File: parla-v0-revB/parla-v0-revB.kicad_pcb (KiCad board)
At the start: 2 copper layers, 80 x 80 mm, 25 parts, among them J1 AudioJack2_SwitchT, J2 AudioJack2_SwitchT, J3 Barrel_Jack_Switch, J4 Barrel_Jack_Switch, J5 AudioJack2_SwitchT, J6 AudioJack2_SwitchT, J7 Conn_01x03_Pin, SW1 SW_SPDT, U1 L7805, U2 PAM8403D

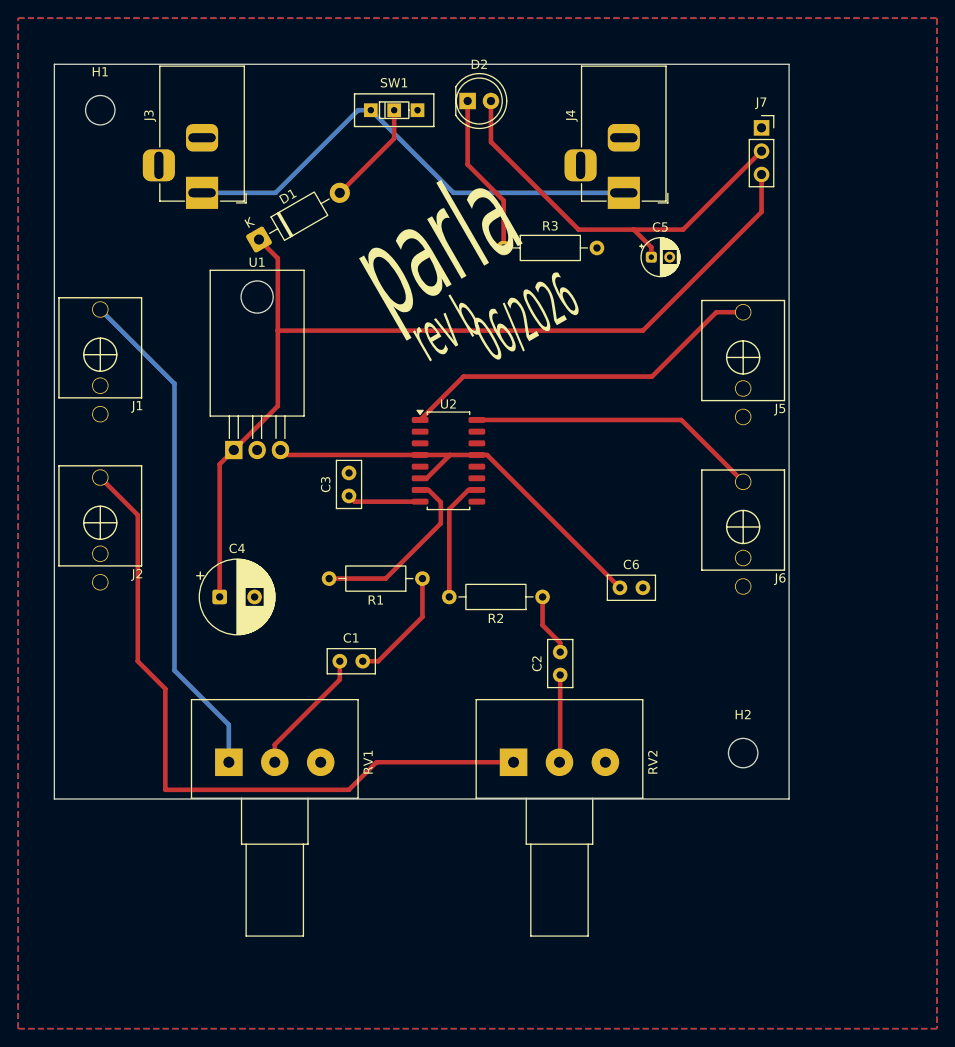
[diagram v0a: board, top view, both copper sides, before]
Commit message: nueva version matias
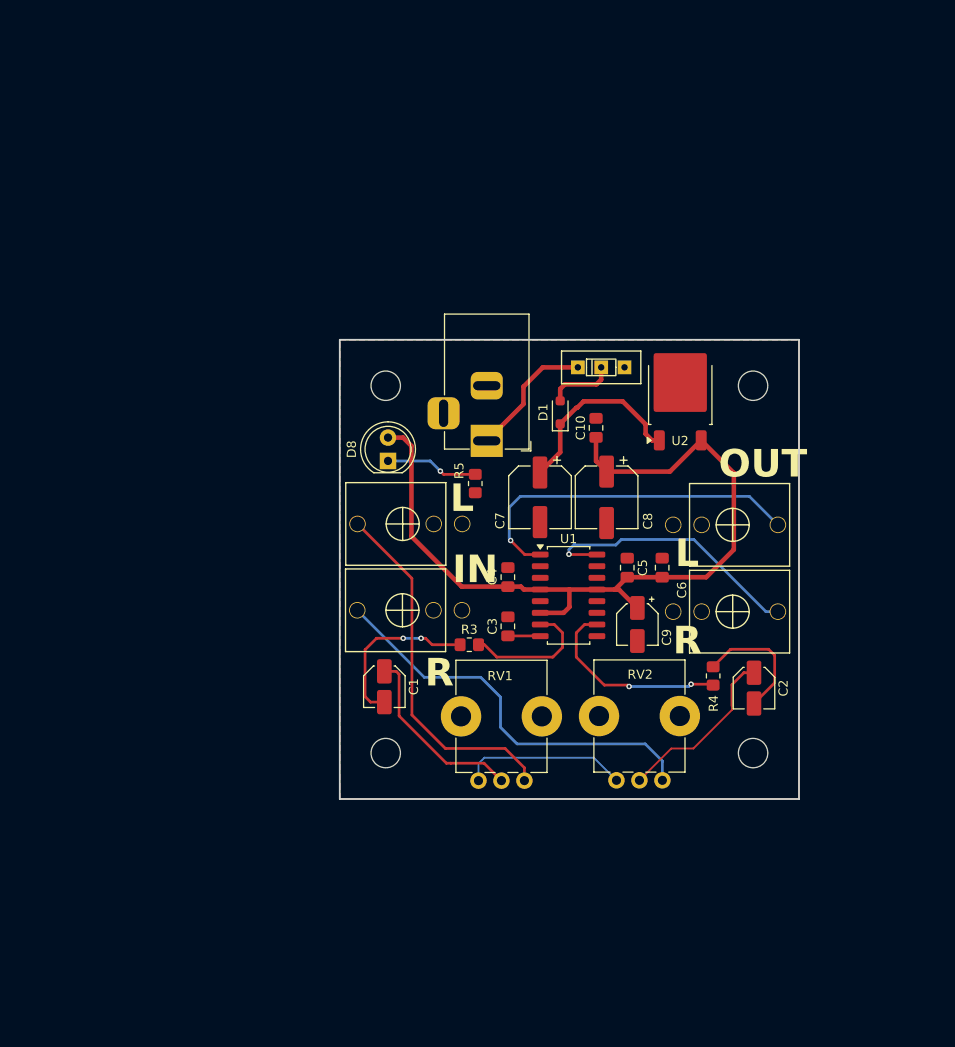
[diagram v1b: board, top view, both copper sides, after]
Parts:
- removed D2: LED, LED_THT:LED_D5.0mm
- removed J6: AudioJack2_SwitchT, parla:PJ301M-12
- removed J7: Conn_01x03_Pin, Connector_PinSocket_2.54mm:PinSocket_1x03_P2.54mm_Vertical
- removed R1, R2: 10k, Resistor_THT:R_Axial_DIN0207_L6.3mm_D2.5mm_P10.16mm_Horizontal
- removed SW1: SW_SPDT, parla:spdt_ssd12d00g3
- added C10: 100n, Capacitor_SMD:C_0805_2012Metric_Pad1.18x1.45mm_HandSolder, F.Cu at (77.9, 59.6)
- added C7: 100u, Capacitor_SMD:CP_Elec_6.3x7.7, F.Cu at (71.8, 67.2)
- added C8: 220u, Capacitor_SMD:CP_Elec_6.3x5.4, F.Cu at (79.0, 67.2)
- added C9: 10u, Capacitor_SMD:CP_Elec_4x5.4, F.Cu at (82.4, 81.0)
- added D8: LED, LED_THT:LED_D5.0mm, F.Cu at (55.2, 63.2)
- added H3: M3, MountingHole:MountingHole_3.2mm_M3, F.Cu at (55.0, 95.0)
- added H4: M3, MountingHole:MountingHole_3.2mm_M3, F.Cu at (95.0, 95.0)
- added R4: 10k, Resistor_SMD:R_0805_2012Metric_Pad1.20x1.40mm_HandSolder, F.Cu at (90.7, 86.6)
- added R5: 1k, Resistor_SMD:R_0805_2012Metric_Pad1.20x1.40mm_HandSolder, F.Cu at (64.8, 65.7)
- added SW3: SW_SPDT, dis8644:spdt_ssd12d00g3, F.Cu at (78.5, 53.0)
- C1, C2: footprint Capacitor_THT:C_Disc_D5.0mm_W2.5mm_P2.50mm -> Capacitor_SMD:C_Elec_4x5.4
- C3: footprint Capacitor_THT:C_Disc_D5.0mm_W2.5mm_P2.50mm -> Capacitor_SMD:C_0805_2012Metric_Pad1.18x1.45mm_HandSolder
- C4: value 100u -> 1u; footprint Capacitor_THT:CP_Radial_D8.0mm_P3.80mm -> Capacitor_SMD:C_0805_2012Metric_Pad1.18x1.45mm_HandSolder
- C5: value 10u -> 1u; footprint Capacitor_THT:CP_Radial_D4.0mm_P2.00mm -> Capacitor_SMD:C_0805_2012Metric_Pad1.18x1.45mm_HandSolder
- C6: value 100n -> 1u; footprint Capacitor_THT:C_Disc_D5.0mm_W2.5mm_P2.50mm -> Capacitor_SMD:C_0805_2012Metric_Pad1.18x1.45mm_HandSolder
- D1: footprint Diode_THT:D_DO-41_SOD81_P10.16mm_Horizontal -> Diode_SMD:D_SOD-323_HandSoldering
- J1, J2: footprint parla:PJ301M-12 -> dis8644:PJ301M-12-T_TN_S
- J3, J4: value Barrel_Jack_Switch -> AudioJack2_SwitchT; footprint Connector_BarrelJack:BarrelJack_Horizontal -> dis8644:PJ301M-12-T_TN_S
- J5: value AudioJack2_SwitchT -> Barrel_Jack_Switch; footprint parla:PJ301M-12 -> Connector_BarrelJack:BarrelJack_Horizontal
- R3: value 1k -> 10k; footprint Resistor_THT:R_Axial_DIN0207_L6.3mm_D2.5mm_P10.16mm_Horizontal -> Resistor_SMD:R_0805_2012Metric_Pad1.20x1.40mm_HandSolder
- RV1, RV2: footprint Potentiometer_THT:Potentiometer_Alps_RK163_Single_Horizontal -> Potentiometer_THT:Potentiometer_Bourns_PTV09A-1_Single_Vertical
- U1: value L7805 -> PAM8403D; footprint Package_TO_SOT_THT:TO-220-3_Horizontal_TabDown -> Package_SO:SOP-16_4.4x10.4mm_P1.27mm
- U2: value PAM8403D -> L7805; footprint Package_SO:SOP-16_4.4x10.4mm_P1.27mm -> Package_TO_SOT_SMD:TO-252-2
- moved J1 71.3 mm to (92.8, 70.2), turned to -90 degrees
- moved J2 69.5 mm to (92.8, 79.6), turned to -90 degrees
- moved J4 51.4 mm to (56.8, 79.5), turned to 90 degrees
- moved R3 43.4 mm to (64.1, 83.2)
- moved H1 43.2 mm to (55.0, 55.0)
- moved J3 42.2 mm to (56.8, 70.0), turned to 90 degrees
- moved H2 40.0 mm to (95.0, 55.0)
- moved U1 39.7 mm to (74.9, 77.8)
- moved D1 37.8 mm to (74.0, 57.9), turned to 90 degrees
- moved C5 33.9 mm to (81.3, 74.8), turned to -90 degrees
- moved RV1 32.2 mm to (70.1, 98.0)
- moved C4 31.5 mm to (68.3, 75.8), turned to -90 degrees
- moved J5 29.4 mm to (66.0, 61.0), turned to -90 degrees
- moved U2 26.3 mm to (87.1, 55.9), turned to 90 degrees
- moved C3 22.4 mm to (68.3, 81.2)
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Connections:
- C3 pad 1: Net-(U2-VREF) -> Net-(U1-VREF)
- C4 pad 1: +12V -> GND
- C4 pad 2: GND -> +5V
- C5 pad 1: +5V -> GND
- C5 pad 2: GND -> +5V
- C6 pad 1: +5V -> GND
- C6 pad 2: GND -> +5V
- J5 pad 1: GND -> Net-(SW3-A)
- J5 pad 2: unconnected-(J5-Pad2) -> GND
- J5 pad 3: Net-(U2-LOUT+) -> unconnected-(J5-Pad3)
- R3 pad 1: Net-(D2-K) -> Net-(C1-Pad2)
- R3 pad 2: GND -> Net-(U1-INL)
- RV1 pad 1: Net-(J1-Pad3) -> Net-(J3-PadT)
- RV2 pad 1: Net-(J2-Pad3) -> Net-(J4-PadT)
- U1 pad 1: +12V -> Net-(U1-LOUT+)
- U1 pad 3: +5V -> GND
- U2 pad 1: Net-(U2-LOUT+) -> +12V
- U2 pad 3: GND -> +5V
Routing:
- net +12V: track 104.5 -> 20.4 mm
- net Net-(J2-Pad3): track 76.1 -> 0.00 mm
- net Net-(J1-Pad3): track 55.1 -> 0.00 mm
- net Net-(SW1-A): track 53.4 -> 0.00 mm
- net Net-(J4-PadT): track 0.00 -> 44.1 mm
- net Net-(U2-LOUT+): track 40.0 -> 0.00 mm
- net Net-(J3-PadT): track 0.00 -> 39.3 mm
- net Net-(U1-LOUT+): track 0.00 -> 38.6 mm, vias 0 -> 1
- net Net-(U2-ROUT+): track 31.8 -> 0.00 mm
- net Net-(U1-ROUT+): track 0.00 -> 30.1 mm, vias 0 -> 1
- net Net-(U1-INR): track 0.00 -> 21.6 mm, vias 0 -> 2
- net Net-(U2-INL): track 19.8 -> 0.00 mm
- net GND: track 0.00 -> 18.2 mm
- net Net-(D2-K): track 17.6 -> 0.00 mm
- net Net-(U1-INL): track 0.00 -> 14.5 mm
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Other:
- board size 80 x 80 mm -> 50 x 50 mm
- board text added: "IN"
- board text added: "L"
- board text added: "OUT"
- board text added: "PARLA"
- board text added: "R"
- board text added: "rev B 06-2026"
- board text removed: "06/2026"
- board text removed: "parla"
- board text removed: "rev b"
